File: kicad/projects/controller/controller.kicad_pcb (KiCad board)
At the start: 2 copper layers, 74 x 40 mm, 56 parts, among them J1 Buttons, J2 Joystick left, J3 Joystick right, J4 Display, J5 18650, J6 Rumble1, J7 Rumble2, J8 ADS1115, J9 LEDs, Q1 DMG2301L, Q2 MMBT2222A, Q3 DMG2301L, SW2 SW_DP3T, U2 ESP32-C6-SUPERMINI, U3 MCP1826T-3302E/DC

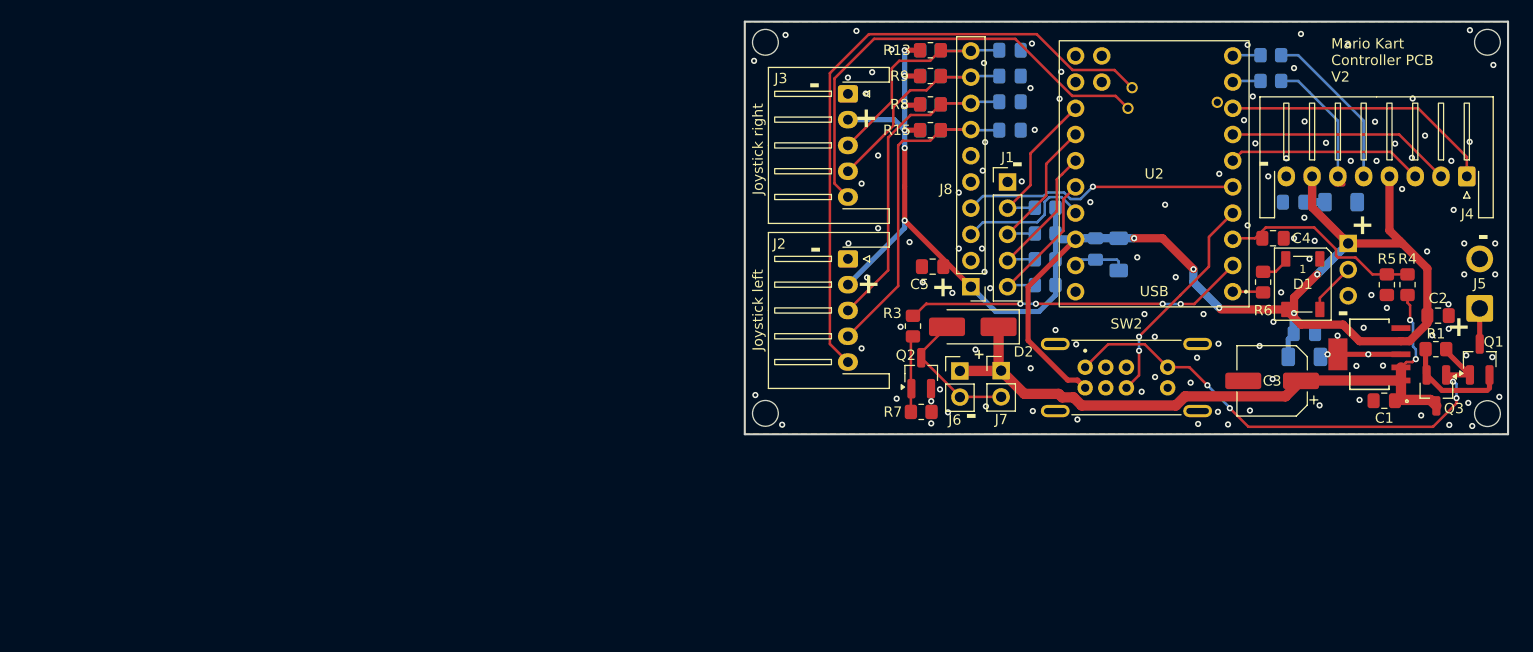
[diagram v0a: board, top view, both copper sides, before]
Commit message: video/ ignorieren (Videos gehen übers Wiki)
Co-Authored-By: Claude Opus 5.5 <noreply@anthropic.com>
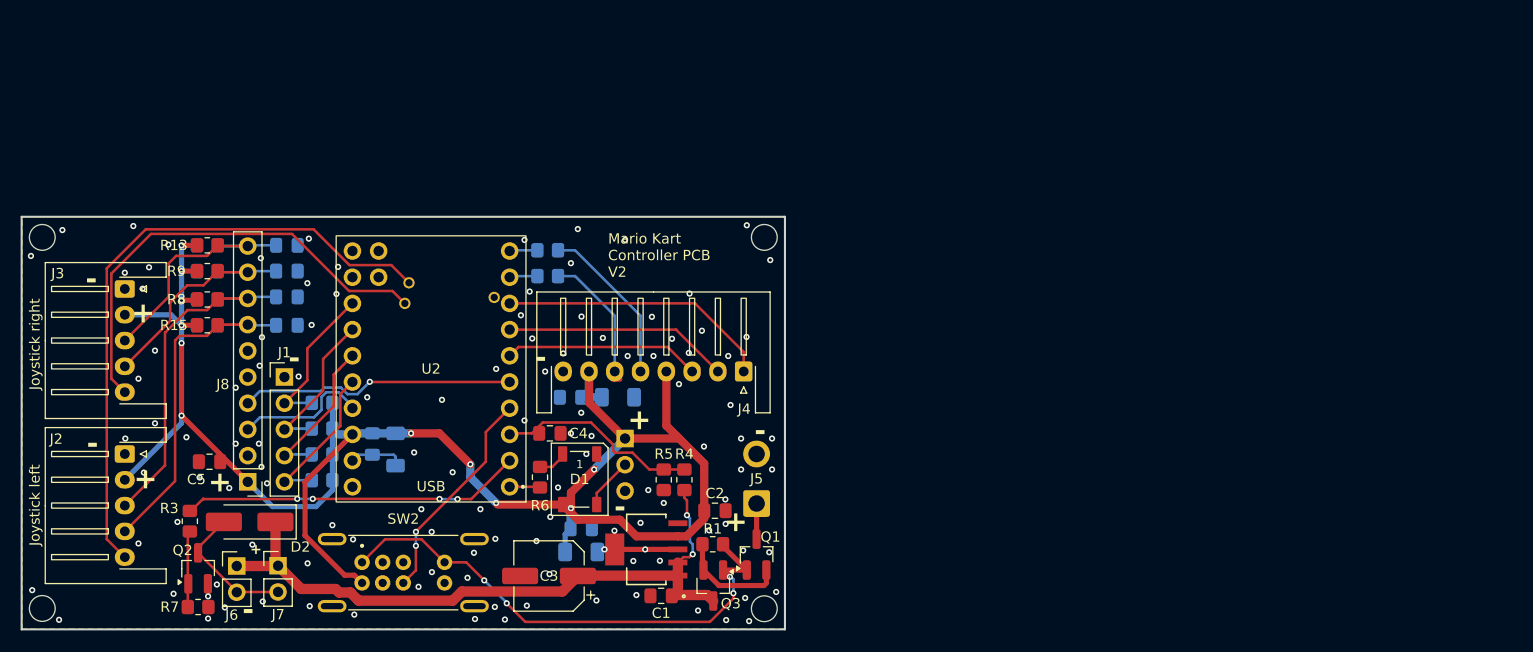
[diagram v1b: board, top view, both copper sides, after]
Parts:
- moved Q3 72.6 mm to (117.4, 86.2)
- moved C1 72.6 mm to (112.4, 87.2)
- moved C10 72.6 mm to (103.6, 67.9)
- moved C11 72.6 mm to (76.1, 60.9)
- moved C12 72.6 mm to (76.1, 58.2)
- moved C13 72.6 mm to (76.1, 55.7)
- moved C14 72.6 mm to (76.1, 53.2)
- moved C15 72.6 mm to (104.6, 82.9)
- moved C2 72.6 mm to (117.6, 78.9)
- moved C3 72.6 mm to (101.5, 85.2)
- moved C4 72.6 mm to (101.6, 71.4)
- moved C5 72.6 mm to (68.6, 74.2)
- moved C6 72.6 mm to (104.6, 80.7)
- moved C7 72.6 mm to (86.6, 73.0)
- moved C8 72.6 mm to (84.4, 72.5)
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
